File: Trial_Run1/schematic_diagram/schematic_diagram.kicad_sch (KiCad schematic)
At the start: 21 parts, among them J1 Power, J2 PWM, J3 Analog, J4 PWM, J5 Analog, J6 Communication, J7 Digital, M1 Motor_Servo, U1 N20_Geared_MicroMotor, U2 QTR-9A, U3 MPU-6050, U4 64 Data ToF Imager, U5 TF-Luna I2C, U6 TF-Luna I2C, U7 MFRC522, U8 N20_Geared_MicroMotor

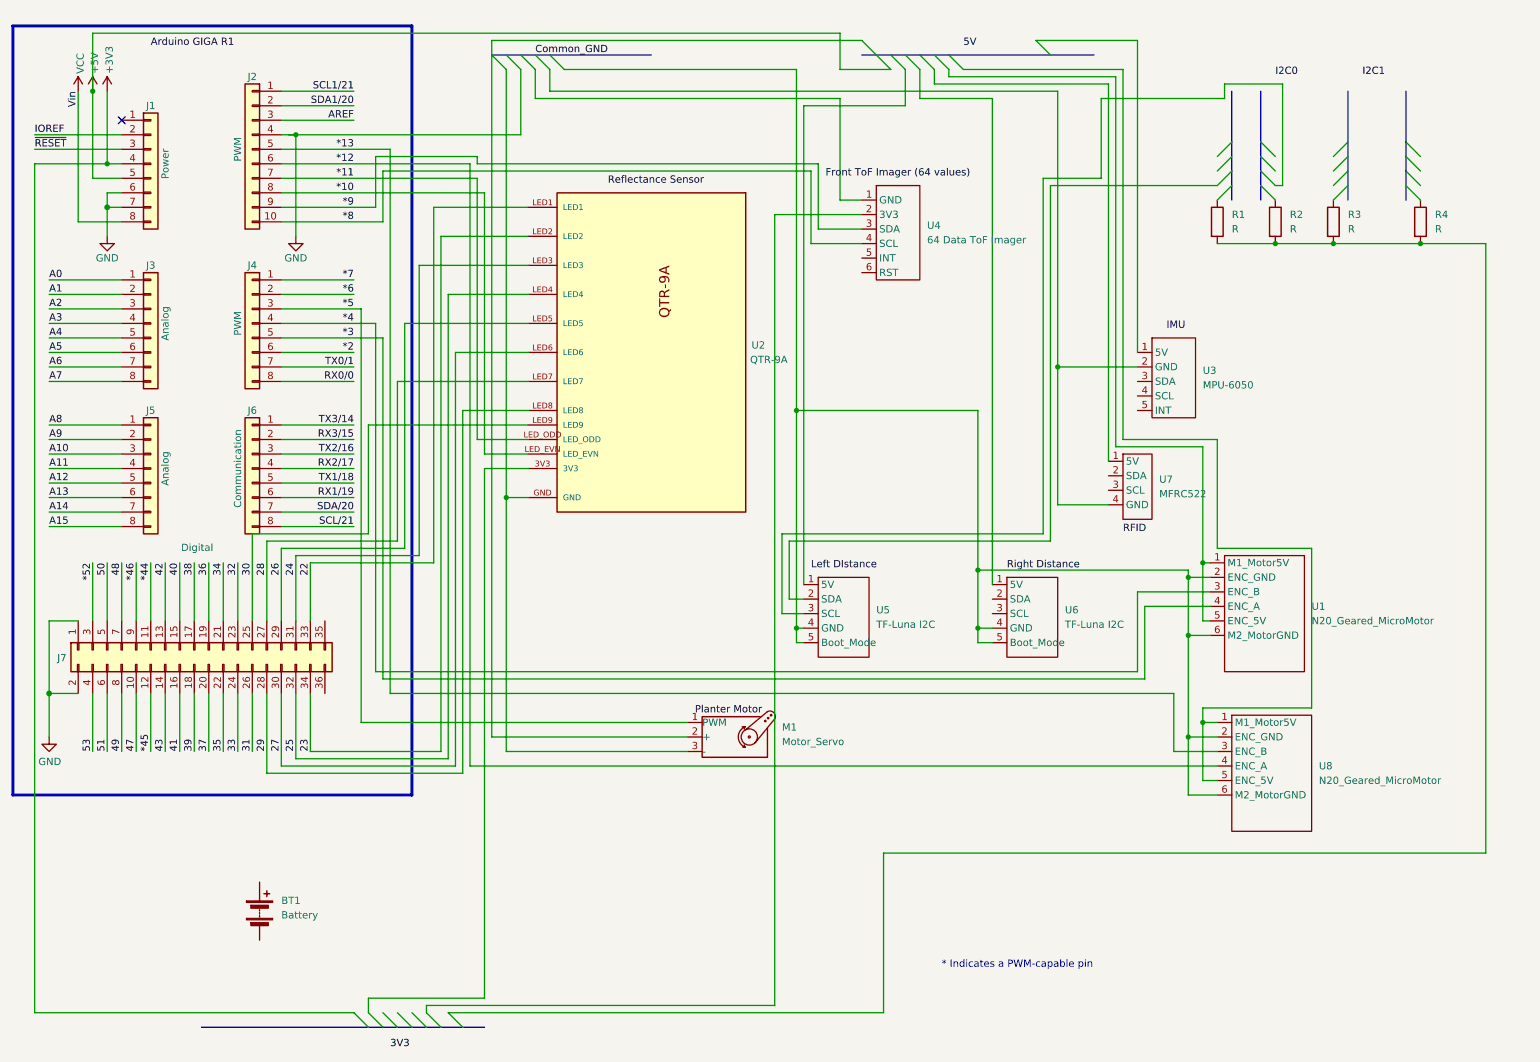
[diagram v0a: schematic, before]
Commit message: working code
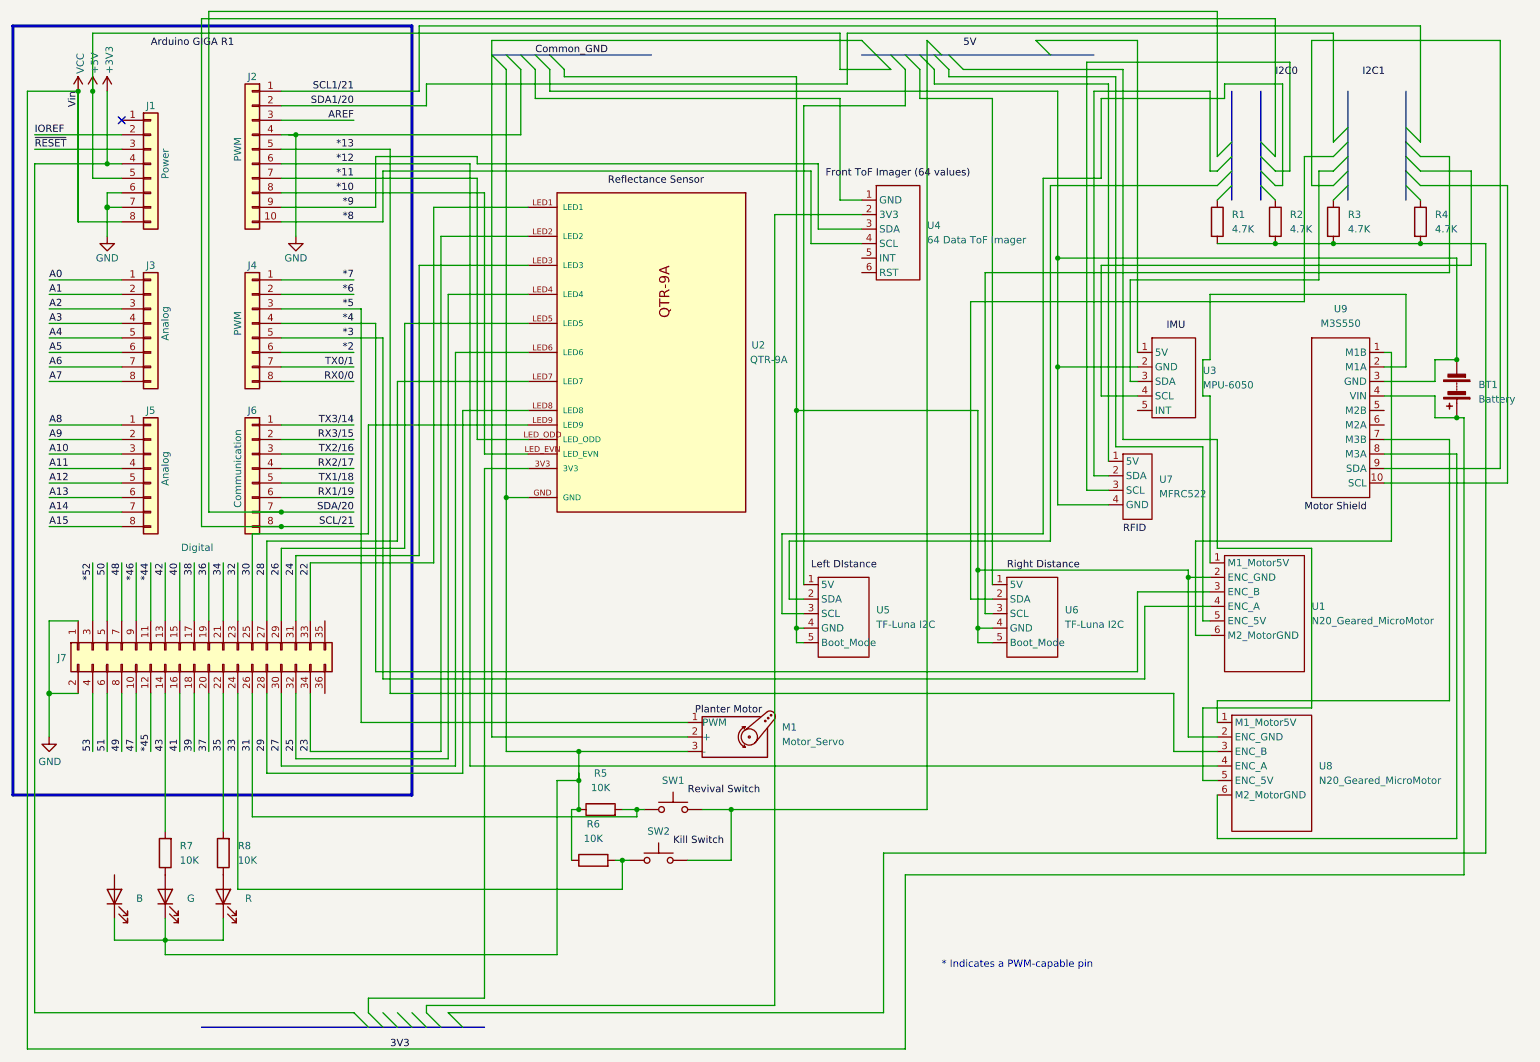
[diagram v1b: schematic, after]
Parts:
- added B, G, R: LED, symbol Device:LED
- added R5, R6, R7, R8: 10K, symbol Device:R
- added SW1, SW2: SW_Push, symbol Switch:SW_Push
- added U9: M3S550, symbol Custom_Stuff:M3S550
- R1, R2, R3, R4: value R -> 4.7K
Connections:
- net SCL/21 is gone; now on net I2C0: J6.8 (Pin_8)
- net 31: now also R5.2, SW1.1
- net 33: now also R6.2, SW2.1
- net 35: now also R8.2
- net 43: now also R7.2
- net Right Distance: no longer U1.6 (M2_MotorGND), U8.6 (M2_MotorGND)
- net VCC: now also BT1.1 (+), U9.4 (VIN)
- net at M1.3 (-), U2.GND: now also B.1 (K), G.1 (K), R.1 (K), R5.1, R6.1
- net at U1.1 (M1_Motor5V): now also U9.2 (M1A); no longer U1.5 (ENC_5V)
- net at BT1.2 (-): now also U3.2 (GND), U7.4 (GND), U9.3 (GND)
- net at U8.1 (M1_Motor5V): now also U9.7 (M3B); no longer U8.5 (ENC_5V)
- new net: G.2 (A), R7.1
- new net: U1.6 (M2_MotorGND), U9.1 (M1B)
- new net: SW1.2, SW2.2
- new net: U8.6 (M2_MotorGND), U9.8 (M3A)
- new net: R.2 (A), R8.1
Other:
- moved on the sheet: BT1
